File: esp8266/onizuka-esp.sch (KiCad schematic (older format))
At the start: 3 parts, among them P1 CONN_01X06, P2 CONN_01X04, P3 CONN_02X04

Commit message: Various upgrades, also ESP-12E footprint for ESP board
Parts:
- removed P1: CONN_01X06, Socket_Strips:Socket_Strip_Angled_1x06, symbol CONN_01X06
- removed P2: CONN_01X04, Socket_Strips:Socket_Strip_Angled_1x04, symbol CONN_01X04
- removed P3: CONN_02X04, Socket_Strips:Socket_Strip_Straight_2x04, symbol CONN_02X04
- added C1, C4: 100n, Capacitors_SMD:C_0603, symbol C_Small
- added C2, C3: 22u, Capacitors_SMD:C_0603, symbol C_Small
- added P1: FTDI, Socket_Strips:Socket_Strip_Angled_2x06, symbol CONN_02X06
- added U1: ESP-01, Socket_Strips:Socket_Strip_Straight_2x04, symbol ESP-01
- added U2: ESP-12E, esp:ESP-12E, symbol ESP-12E
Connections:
- net labels removed: GPIO2
- wire segments 5 -> 13
- no-connect marks 0 -> 22

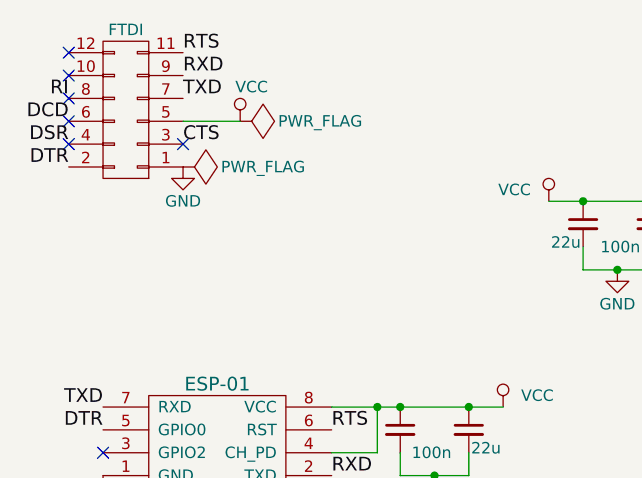
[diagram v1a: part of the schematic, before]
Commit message: Various tweaks
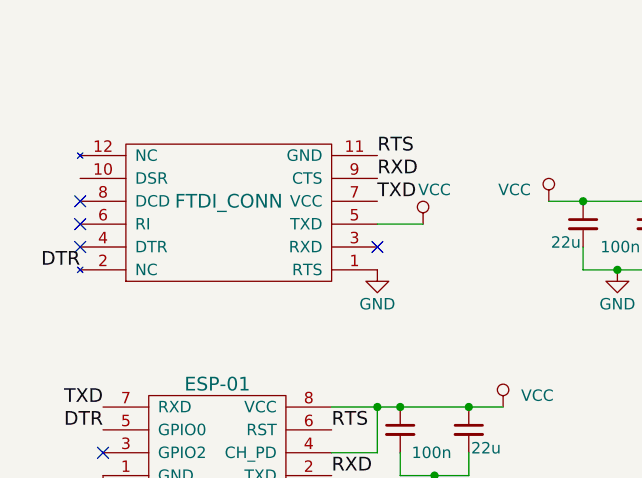
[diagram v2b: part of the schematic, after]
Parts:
- removed P1: FTDI, Socket_Strips:Socket_Strip_Angled_2x06, symbol CONN_02X06
- added C5: FTDI_CONN, Socket_Strips:Socket_Strip_Angled_2x06, symbol FTDI_CONN
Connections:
- net DTR: now also C5.2 (NC)
- net GND: now also C5.1 (RTS)
- net RTS: now also C5.11 (GND)
- net RXD: now also C5.9 (CTS)
- net TXD: now also C5.7 (VCC)
- net VCC: now also C5.5 (TXD)
- no-connect marks 22 -> 20
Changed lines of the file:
@@
 LIBS:valves
 LIBS:esp
+LIBS:onizuka
 LIBS:onizuka-esp-cache
 EELAYER 25 0
@@
 $EndDescr
 $Comp
-L GND #PWR2
+L GND #PWR01
 U 1 1 57423885
-P 1150 1150
-F 0 "#PWR2" H 1150 900 50  0001 C CNN
-F 1 "GND" H 1150 1000 50  0000 C CNN
-F 2 "" H 1150 1150 50  0000 C CNN
-F 3 "" H 1150 1150 50  0000 C CNN
-	1    1150 1150
-	1    0    0    -1
-$EndComp
-$Comp
-L PWR_FLAG #FLG1
-U 1 1 574238B1
-P 1150 1150
-F 0 "#FLG1" H 1150 1245 50  0001 C CNN
-F 1 "PWR_FLAG" V 1150 1500 50  0000 C CNN
-F 2 "" H 1150 1150 50  0000 C CNN
-F 3 "" H 1150 1150 50  0000 C CNN
-	1    1150 1150
-	0    1    1    0
-$EndComp
-$Comp
-L VCC #PWR3
+P 2000 1600
+F 0 "#PWR01" H 2000 1350 50  0001 C CNN
+F 1 "GND" H 2000 1450 50  0000 C CNN
+F 2 "" H 2000 1600 50  0000 C CNN
+F 3 "" H 2000 1600 50  0000 C CNN
+	1    2000 1600
+	1    0    0    -1
+$EndComp
+$Comp
+L VCC #PWR02
 U 1 1 574238E4
-P 1400 950
-F 0 "#PWR3" H 1400 800 50  0001 C CNN
-F 1 "VCC" H 1450 1100 50  0000 C CNN
-F 2 "" H 1400 950 50  0000 C CNN
-F 3 "" H 1400 950 50  0000 C CNN
-	1    1400 950
-	1    0    0    -1
-$EndComp
-Text Label 1150 1050 0    60   ~ 0
-CTS
-Wire Wire Line
-	1400 950  1150 950
-Text Label 1150 850  0    60   ~ 0
+P 2200 1400
+F 0 "#PWR02" H 2200 1250 50  0001 C CNN
+F 1 "VCC" H 2250 1550 50  0000 C CNN
+F 2 "" H 2200 1400 50  0000 C CNN
+F 3 "" H 2200 1400 50  0000 C CNN
+	1    2200 1400
+	1    0    0    -1
+$EndComp
+Text Label 2000 1300 0    60   ~ 0
 TXD
-Text Label 1150 750  0    60   ~ 0
+Text Label 2000 1200 0    60   ~ 0
 RXD
-Text Label 1150 650  0    60   ~ 0
+Text Label 2000 1100 0    60   ~ 0
 RTS
-Text Label 650  1150 2    60   ~ 0
+Text Label 700  1600 2    60   ~ 0
 DTR
-Text Label 650  1050 2    60   ~ 0
-DSR
-Text Label 650  950  2    60   ~ 0
-DCD
-Text Label 650  850  2    60   ~ 0
-RI
 Text Label 1800 2500 0    60   ~ 0
 RXD
@@
 TXD
 $Comp
-L VCC #PWR5
+L VCC #PWR03
 U 1 1 5742AE0A
 P 2550 2200
-F 0 "#PWR5" H 2550 2050 50  0001 C CNN
+F 0 "#PWR03" H 2550 2050 50  0001 C CNN
 F 1 "VCC" H 2700 2250 50  0000 C CNN
 F 2 "" H 2550 2200 50  0000 C CNN
@@
 $EndComp
 $Comp
-L GND #PWR1
+L GND #PWR04
 U 1 1 5742AE21
 P 800 2500
-F 0 "#PWR1" H 800 2250 50  0001 C CNN
+F 0 "#PWR04" H 800 2250 50  0001 C CNN
 F 1 "GND" H 800 2350 50  0000 C CNN
 F 2 "" H 800 2500 50  0000 C CNN
@@
 Text Label 1800 2300 0    60   ~ 0
 RTS
-$Comp
-L PWR_FLAG #FLG2
-U 1 1 5742B0BE
-P 1400 950
-F 0 "#FLG2" H 1400 1045 50  0001 C CNN
-F 1 "PWR_FLAG" V 1400 1300 50  0000 C CNN
-F 2 "" H 1400 950 50  0000 C CNN
-F 3 "" H 1400 950 50  0000 C CNN
-	1    1400 950
-	0    1    1    0
-$EndComp
-$Comp
-L CONN_02X06 P1
-U 1 1 5744C15C
-P 900 900
-F 0 "P1" H 900 1250 50  0001 C CNN
-F 1 "FTDI" H 900 550 50  0000 C CNN
-F 2 "Socket_Strips:Socket_Strip_Angled_2x06" H 900 -300 50  0001 C CNN
-F 3 "" H 900 -300 50  0000 C CNN
-	1    900  900
-	-1   0    0    1
-$EndComp
-NoConn ~ 650  850
-NoConn ~ 650  950
-NoConn ~ 650  1050
-NoConn ~ 1150 1050
 $Comp
 L C_Small C1
@@
 	2400 2500 2400 2400
 $Comp
-L GND #PWR4
+L GND #PWR05
 U 1 1 5744C48B
 P 2250 2500
-F 0 "#PWR4" H 2250 2250 50  0001 C CNN
+F 0 "#PWR05" H 2250 2250 50  0001 C CNN
 F 1 "GND" H 2250 2350 50  0000 C CNN
 F 2 "" H 2250 2500 50  0000 C CNN
@@
 $EndComp
 Connection ~ 2250 2500
-NoConn ~ 650  750
-NoConn ~ 650  650
 $Comp
 L ESP-01 U1
@@
 RTS
 $Comp
-L VCC #PWR6
+L VCC #PWR06
 U 1 1 5744F3A3
 P 2750 1300
-F 0 "#PWR6" H 2750 1150 50  0001 C CNN
+F 0 "#PWR06" H 2750 1150 50  0001 C CNN
 F 1 "VCC" H 2900 1350 50  0000 C CNN
 F 2 "" H 2750 1300 50  0000 C CNN
@@
 	2900 1600 2900 1500
 $Comp
-L GND #PWR7
+L GND #PWR07
 U 1 1 5744F3BB
 P 3050 1600
-F 0 "#PWR7" H 3050 1350 50  0001 C CNN
+F 0 "#PWR07" H 3050 1350 50  0001 C CNN
 F 1 "GND" H 3050 1450 50  0000 C CNN
 F 2 "" H 3050 1600 50  0000 C CNN
@@
 	3300 1800 3500 1800
 $Comp
-L GND #PWR8
+L GND #PWR08
 U 1 1 5744F416
 P 5200 1800
-F 0 "#PWR8" H 5200 1550 50  0001 C CNN
+F 0 "#PWR08" H 5200 1550 50  0001 C CNN
 F 1 "GND" H 5200 1650 50  0000 C CNN
 F 2 "" H 5200 1800 50  0000 C CNN
@@
 NoConn ~ 5200 1400
 NoConn ~ 5200 1300
+$Comp
+L FTDI_CONN C5
+U 1 1 574E1B8D
+P 1350 1350
+F 0 "C5" H 1350 1000 60  0001 C CNN
+F 1 "FTDI_CONN" H 1350 1400 60  0000 C CNN
+F 2 "Socket_Strips:Socket_Strip_Angled_2x06" H 1350 1350 60  0001 C CNN
+F 3 "" H 1350 1350 60  0000 C CNN
+	1    1350 1350
+	1    0    0    -1
+$EndComp
+Wire Wire Line
+	2200 1400 2000 1400
+NoConn ~ 2000 1500
+NoConn ~ 700  1500
+NoConn ~ 700  1300
+NoConn ~ 700  1400
 $EndSCHEMATC

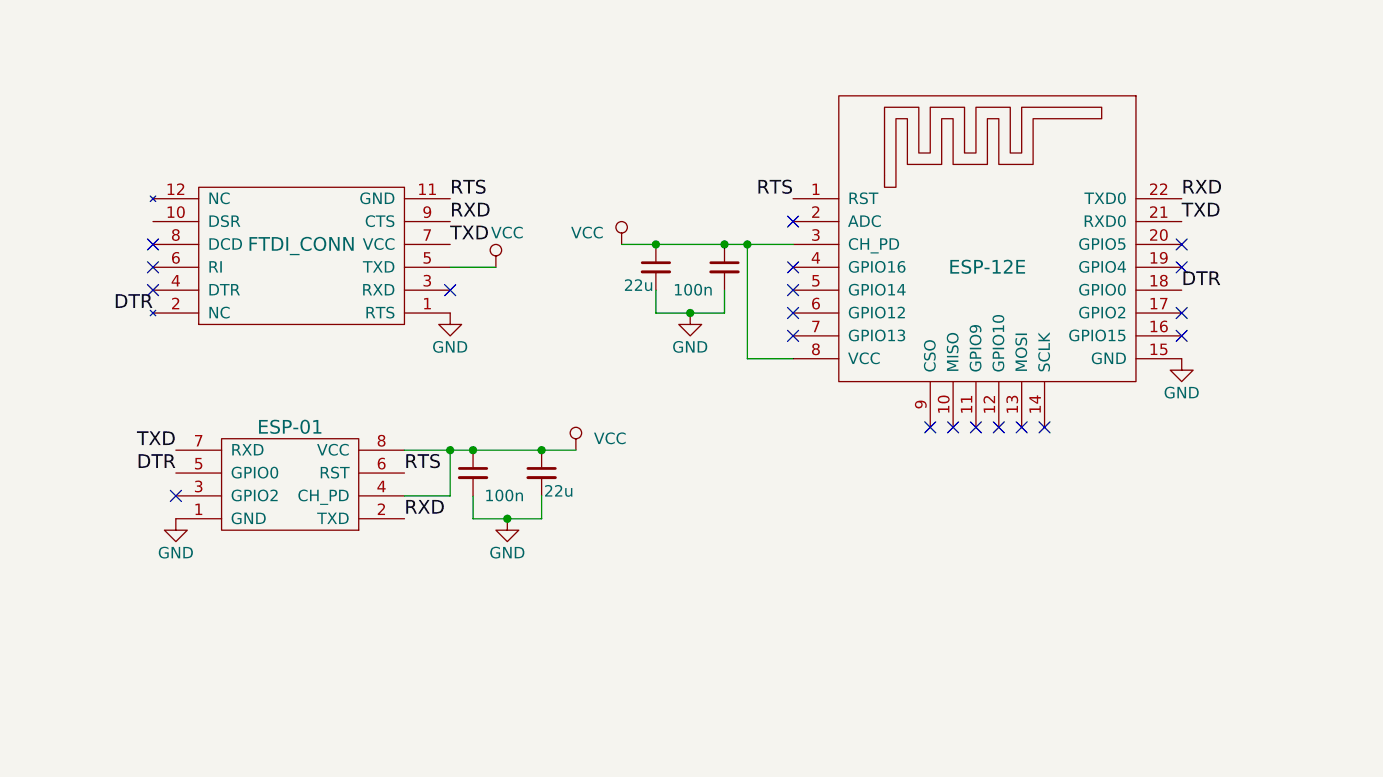
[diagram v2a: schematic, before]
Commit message: Many faffing, new ESP stuff.
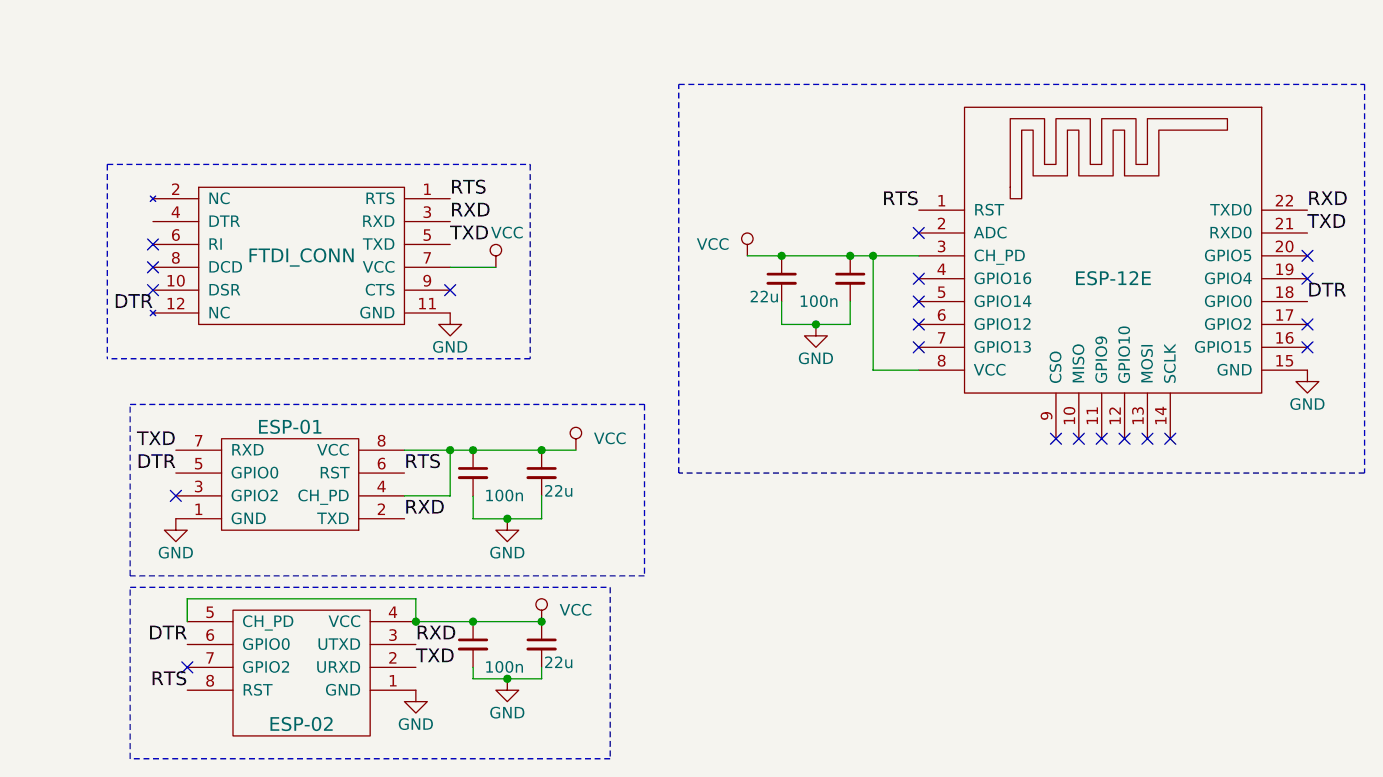
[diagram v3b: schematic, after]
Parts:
- removed C5: FTDI_CONN, Socket_Strips:Socket_Strip_Angled_2x06, symbol FTDI_CONN
- added C6: 100n, Capacitors_SMD:C_0603, symbol C_Small
- added C7: 22u, Capacitors_SMD:C_0603, symbol C_Small
- added P1: FTDI_CONN, Pin_Headers:Pin_Header_Angled_2x06, symbol FTDI_CONN
- added U3: ESP-02, ESP:ESP-02-Program, symbol ESP-02
- U2: footprint esp:ESP-12E -> ESP:ESP-12E-Program
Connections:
- net DTR: now also P1.12 (NC), U3.6 (GPIO0)
- net GND: now also C6.2, C7.2, P1.11 (GND), U3.1 (GND)
- net RTS: now also P1.1 (RTS), U3.8 (RST)
- net RXD: now also P1.3 (RXD), U3.3 (UTXD)
- net TXD: now also P1.5 (TXD), U3.2 (URXD)
- net VCC: now also C6.1, C7.1, P1.7 (VCC), U3.4 (VCC), U3.5 (CH_PD)
- no-connect marks 20 -> 21

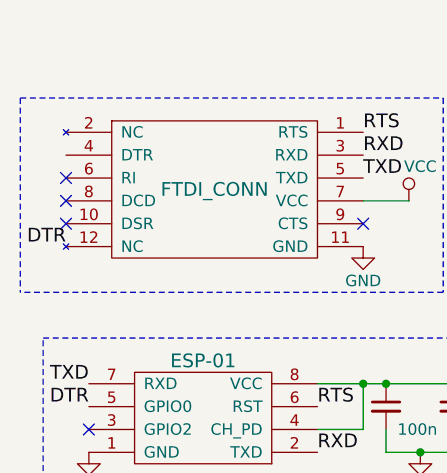
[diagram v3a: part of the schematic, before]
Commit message: Various shuffling, adding farnell part numbers.
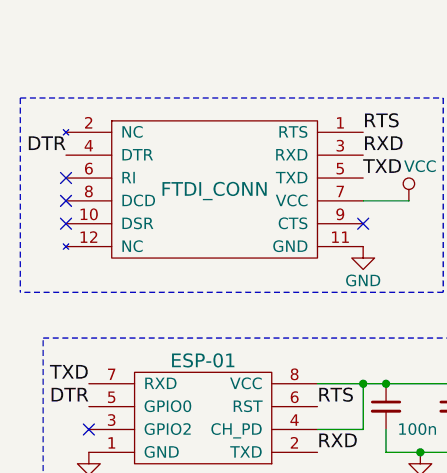
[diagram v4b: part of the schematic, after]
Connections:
- net DTR: now also P1.4 (DTR); no longer P1.12 (NC)
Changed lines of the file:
@@
 Text Label 2000 1100 0    60   ~ 0
 RTS
-Text Label 700  1600 2    60   ~ 0
+Text Label 700  1200 2    60   ~ 0
 DTR
 Text Label 1800 2500 0    60   ~ 0
@@
 $Comp
 L FTDI_CONN P1
-U 1 1 5750541E
+U 1 1 5750A0BC
 P 1350 1350
 F 0 "P1" H 1350 863 60  0001 C CNN

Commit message: Final tweaks, more farnell part numbers, BOM, gerbers
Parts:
- C1, C4, C6: Farnell (none) -> 2524817
- C2, C3, C7: Farnell (none) -> 2494232
- P1: Farnell (none) -> 1593452
- U1: footprint Socket_Strips:Socket_Strip_Straight_2x04 -> ESP:ESP-01; Farnell (none) -> 1593489
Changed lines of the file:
@@
 F 1 "100n" H 2150 2200 50  0000 L CNN
 F 2 "Capacitors_SMD:C_0603" H 2100 2300 50  0001 C CNN
-F 3 "" H 2100 2300 50  0000 C CNN
+F 3 "http://www.farnell.com/datasheets/2009679.pdf" H 2100 2300 50  0001 C CNN
+F 4 "2524817" H 2100 2300 60  0001 C CNN "Farnell"
 	1    2100 2300
 	1    0    0    -1
@@
 F 2 "Capacitors_SMD:C_0603" H 2400 2300 50  0001 C CNN
 F 3 "" H 2400 2300 50  0000 C CNN
+F 4 "2494232" H 2400 2300 60  0001 C CNN "Farnell"
 	1    2400 2300
 	1    0    0    -1
@@
 F 0 "U1" H 1300 2100 60  0001 C CNN
 F 1 "ESP-01" H 1300 2600 60  0000 C CNN
-F 2 "Socket_Strips:Socket_Strip_Straight_2x04" H 1300 2550 60  0001 C CNN
+F 2 "ESP:ESP-01" H 1300 2550 60  0001 C CNN
 F 3 "" H 1300 2550 60  0000 C CNN
+F 4 "1593489" H 1300 2350 60  0001 C CNN "Farnell"
 	1    1300 2350
 	1    0    0    -1
@@
 F 2 "Capacitors_SMD:C_0603" H 3750 1450 50  0001 C CNN
 F 3 "" H 3750 1450 50  0000 C CNN
+F 4 "2524817" H 3750 1450 60  0001 C CNN "Farnell"
 	1    3750 1450
 	-1   0    0    -1
@@
 F 2 "Capacitors_SMD:C_0603" H 3450 1450 50  0001 C CNN
 F 3 "" H 3450 1450 50  0000 C CNN
+F 4 "2494232" H 3450 1450 60  0001 C CNN "Farnell"
 	1    3450 1450
 	-1   0    0    -1
@@
 F 2 "Capacitors_SMD:C_0603" H 2100 3050 50  0001 C CNN
 F 3 "" H 2100 3050 50  0000 C CNN
+F 4 "2524817" H 2100 3050 60  0001 C CNN "Farnell"
 	1    2100 3050
 	1    0    0    -1
@@
 F 2 "Capacitors_SMD:C_0603" H 2400 3050 50  0001 C CNN
 F 3 "" H 2400 3050 50  0000 C CNN
+F 4 "2494232" H 2400 3050 60  0001 C CNN "Farnell"
 	1    2400 3050
 	1    0    0    -1
@@
 F 2 "Pin_Headers:Pin_Header_Angled_2x06" H 1250 900 60  0001 C CNN
 F 3 "" H 1350 1350 60  0000 C CNN
+F 4 "1593452" H 1350 1350 60  0001 C CNN "Farnell"
 	1    1350 1350
 	1    0    0    1
